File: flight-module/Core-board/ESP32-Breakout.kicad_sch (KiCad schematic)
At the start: 14 parts, among them J2 USB_B_Micro, SW2 SW_MEC_5E, SW3 SW_MEC_5E, U1 ESP32-S3-WROOM-1-N16R2, U4 AZ1084-3.3

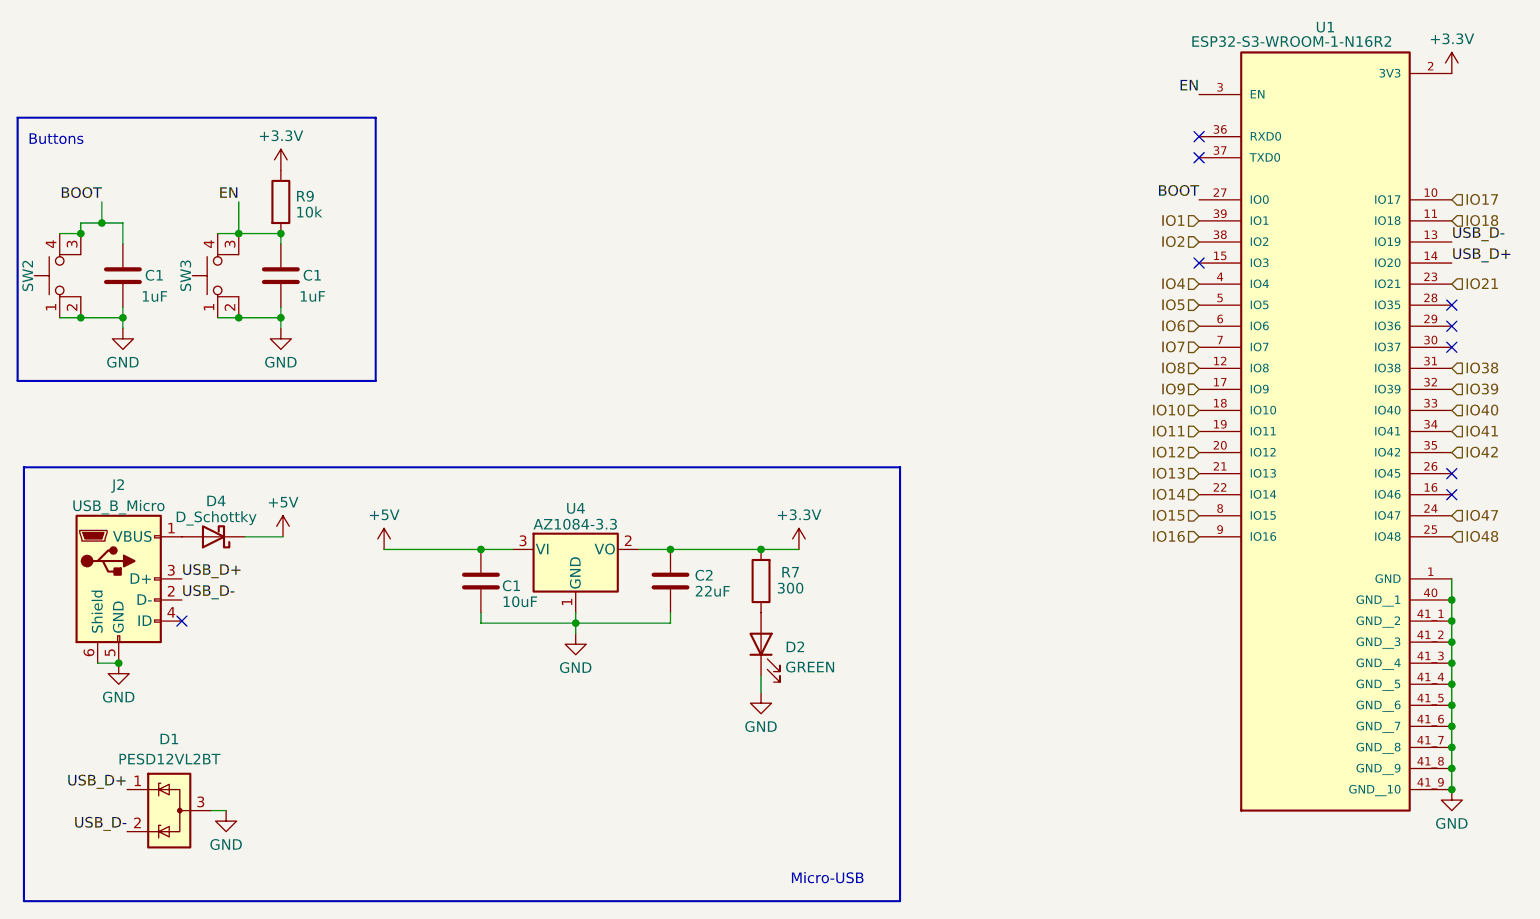
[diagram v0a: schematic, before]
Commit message: Progress on core board.
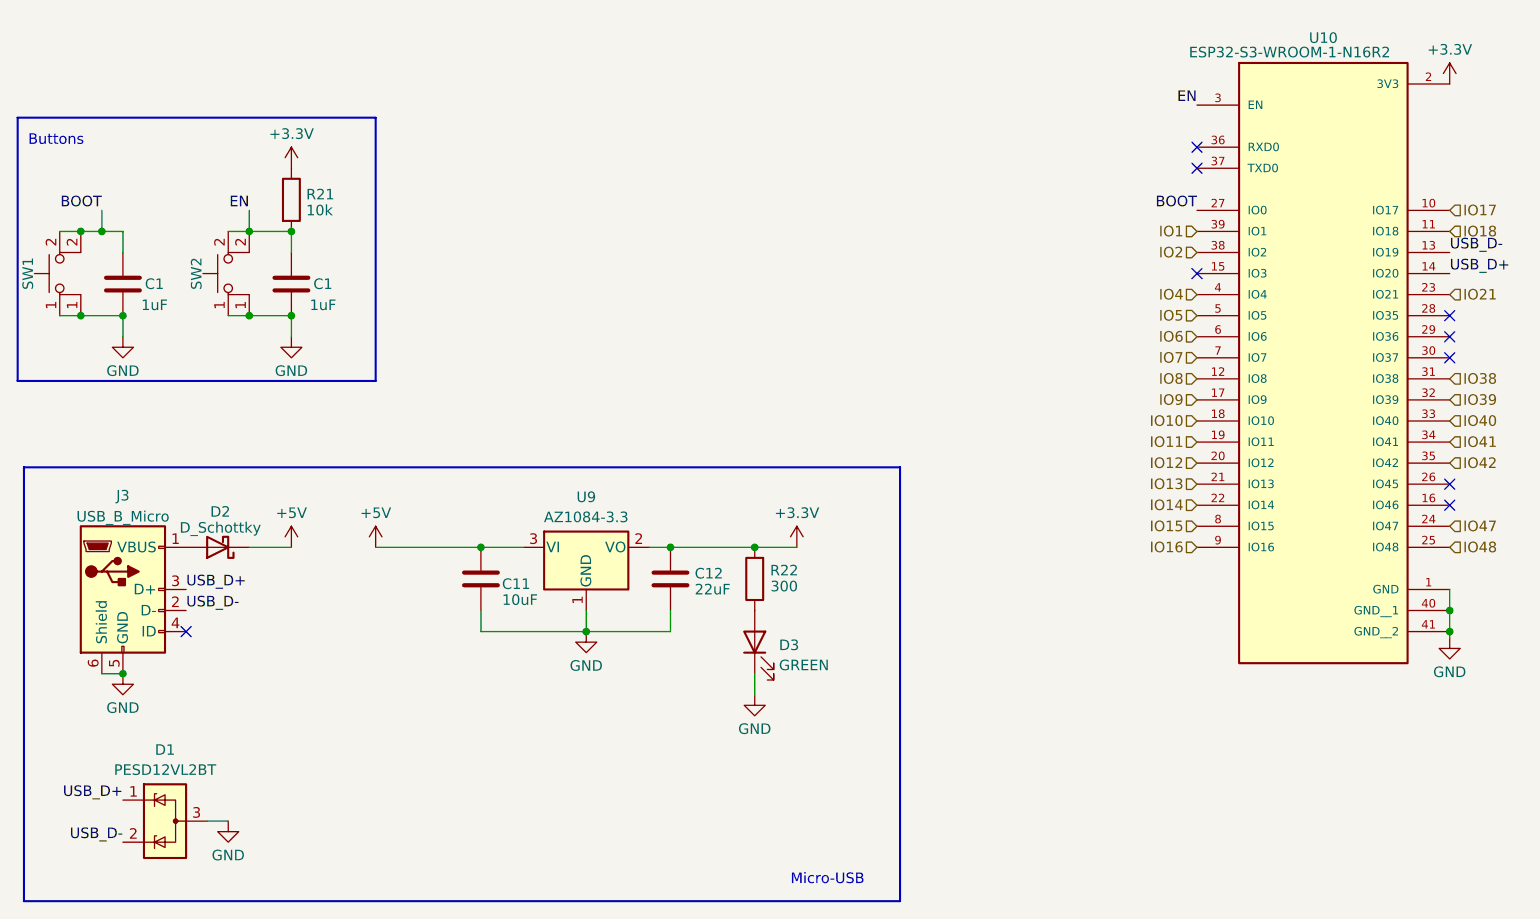
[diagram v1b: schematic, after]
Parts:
- removed SW3: SW_MEC_5E, SnapEDA Library:SW_TS02-66-60-BK-100-SCR-D, symbol Switch:SW_MEC_5E
- added SW2: SW_MEC_5E, Button_Switch_SMD:SW_SPST_TL3305A, symbol Switch:SW_MEC_5E
- J3: renamed from J2; footprint (none) -> Connector_USB:USB_Micro-B_Amphenol_10103594-0001LF_Horizontal
- SW1: renamed from SW2; footprint SnapEDA Library:SW_TS02-66-60-BK-100-SCR-D -> Button_Switch_SMD:SW_SPST_TL3305A
- renumbered C1 to C11, C2 to C12, D4 to D2, D2 to D3, R9 to R21, R7 to R22, U1 to U10, U4 to U9
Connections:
- net BOOT: now also SW1.2; no longer SW1.3 (K), SW1.4 (A)
- net EN: now also SW2.2
- net GND: now also U10.41 (GND__2), SW2.1; no longer SW1.2, U10.41_1 (GND__2), U10.41_2 (GND__3), U10.41_3 (GND__4), U10.41_4 (GND__5), U10.41_5 (GND__6), U10.41_6 (GND__7), U10.41_7 (GND__8), U10.41_8 (GND__9), U10.41_9 (GND__10)
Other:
- moved on the sheet: C1, D1, D2, D3, J3, R21, R22, U9
